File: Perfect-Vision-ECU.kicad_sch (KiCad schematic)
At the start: 13 parts, among them J11 Boot, J5 USB_C_Receptacle_USB2.0_16P, J8 Reset, U2 ESP32-S3-MINI-1

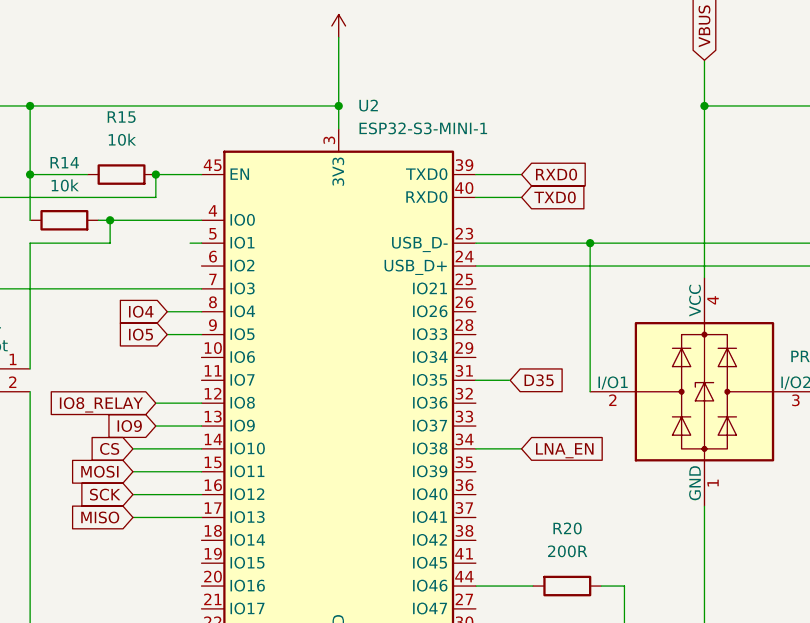
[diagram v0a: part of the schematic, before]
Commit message: Fixes 20/10/2026
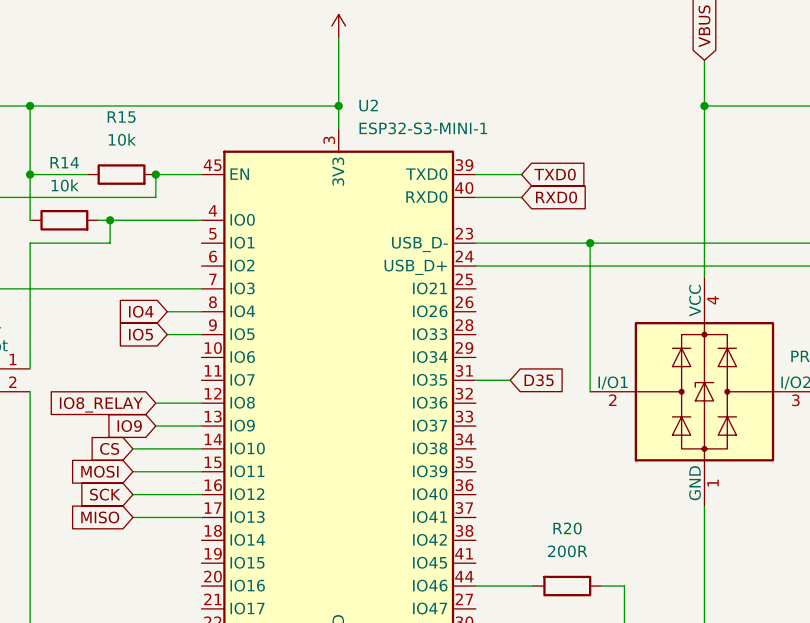
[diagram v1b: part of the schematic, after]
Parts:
- D7: now in the parts list
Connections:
- net RXD0: now also U2.40 (RXD0); no longer U2.39 (TXD0)
- net TXD0: now also U2.39 (TXD0); no longer U2.40 (RXD0)
- net LNA_EN: no longer names the net of U2.34 (IO38)
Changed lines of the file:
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@@
-	(wire
-		(pts
-			(xy 63.5 69.85) (xy 64.77 69.85)
-		)
-		(stroke
-			(width 0)
-			(type default)
-		)
-	)
 	(wire
 		(pts
@@
 		(pts
 			(xy 157.48 66.04) (xy 158.75 66.04)
-		)
-		(stroke
-			(width 0)
-			(type default)
-		)
-	)
-	(wire
-		(pts
-			(xy 95.25 92.71) (xy 100.33 92.71)
 		)
 		(stroke
@@
 		)
 	)
+	(global_label "TXD0"
+		(shape input)
+		(at 100.33 62.23 0)
+		(fields_autoplaced yes)
+		(effects
+			(font
+				(size 1.27 1.27)
+			)
+			(justify left)
+		)
+		(property "Intersheetrefs" "${INTERSHEET_REFS}"
+			(at 108.0669 62.23 0)
+			(effects
+				(font
+					(size 1.27 1.27)
+				)
+				(justify left)
+				(hide yes)
+			)
+		)
+	)
 	(global_label "MOSI"
 		(shape input)
@@
 		)
 	)
-	(global_label "RXD0"
+	(global_label "IO5"
 		(shape input)
-		(at 100.33 62.23 0)
+		(at 60.96 80.01 180)
 		(fields_autoplaced yes)
 		(effects
@@
 				(size 1.27 1.27)
 			)
-			(justify left)
+			(justify right)
 		)
 		(property "Intersheetrefs" "${INTERSHEET_REFS}"
-			(at 108.3693 62.23 0)
-			(effects
-				(font
-					(size 1.27 1.27)
-				)
-				(justify left)
-				(hide yes)
-			)
-		)
-	)
-	(global_label "LNA_EN"
+			(at 54.83 80.01 0)
+			(effects
+				(font
+					(size 1.27 1.27)
+				)
+				(justify right)
+				(hide yes)
+			)
+		)
+	)
+	(global_label "RXD0"
 		(shape input)
-		(at 100.33 92.71 0)
+		(at 100.33 64.77 0)
 		(fields_autoplaced yes)
 		(effects
@@
 		)
 		(property "Intersheetrefs" "${INTERSHEET_REFS}"
-			(at 110.3046 92.71 0)
-			(effects
-				(font
-					(size 1.27 1.27)
-				)
-				(justify left)
-				(hide yes)
-			)
-		)
-	)
-	(global_label "IO5"
-		(shape input)
-		(at 60.96 80.01 180)
-		(fields_autoplaced yes)
-		(effects
-			(font
-				(size 1.27 1.27)
-			)
-			(justify right)
-		)
-		(property "Intersheetrefs" "${INTERSHEET_REFS}"
-			(at 54.83 80.01 0)
-			(effects
-				(font
-					(size 1.27 1.27)
-				)
-				(justify right)
-				(hide yes)
-			)
-		)
-	)
-	(global_label "TXD0"
-		(shape input)
-		(at 100.33 64.77 0)
-		(fields_autoplaced yes)
-		(effects
-			(font
-				(size 1.27 1.27)
-			)
-			(justify left)
-		)
-		(property "Intersheetrefs" "${INTERSHEET_REFS}"
-			(at 108.0669 64.77 0)
+			(at 108.3693 64.77 0)
 			(effects
 				(font
@@
 		(unit 1)
 		(exclude_from_sim no)
-		(in_bom no)
+		(in_bom yes)
 		(on_board yes)
 		(dnp no)
